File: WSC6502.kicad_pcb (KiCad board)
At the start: 2 copper layers, 145.6 x 157 mm, 43 parts, among them IC1 W65C02S6TPG-14 CPU, IC2 AT28C256-15PU ROM, IC3 AS6C62256-55PCN SRAM, IC4 W65C22S6TPG-14 I/O, J1 +5V, J2 +5V, J3 Address Bus, J4 Data Bus, J5 R~W~ TP, J6 , SW1 Reset, SW2 , SW3 , SW4 , SW5 , SW6 , U1 74HC00, Y1 1MHz

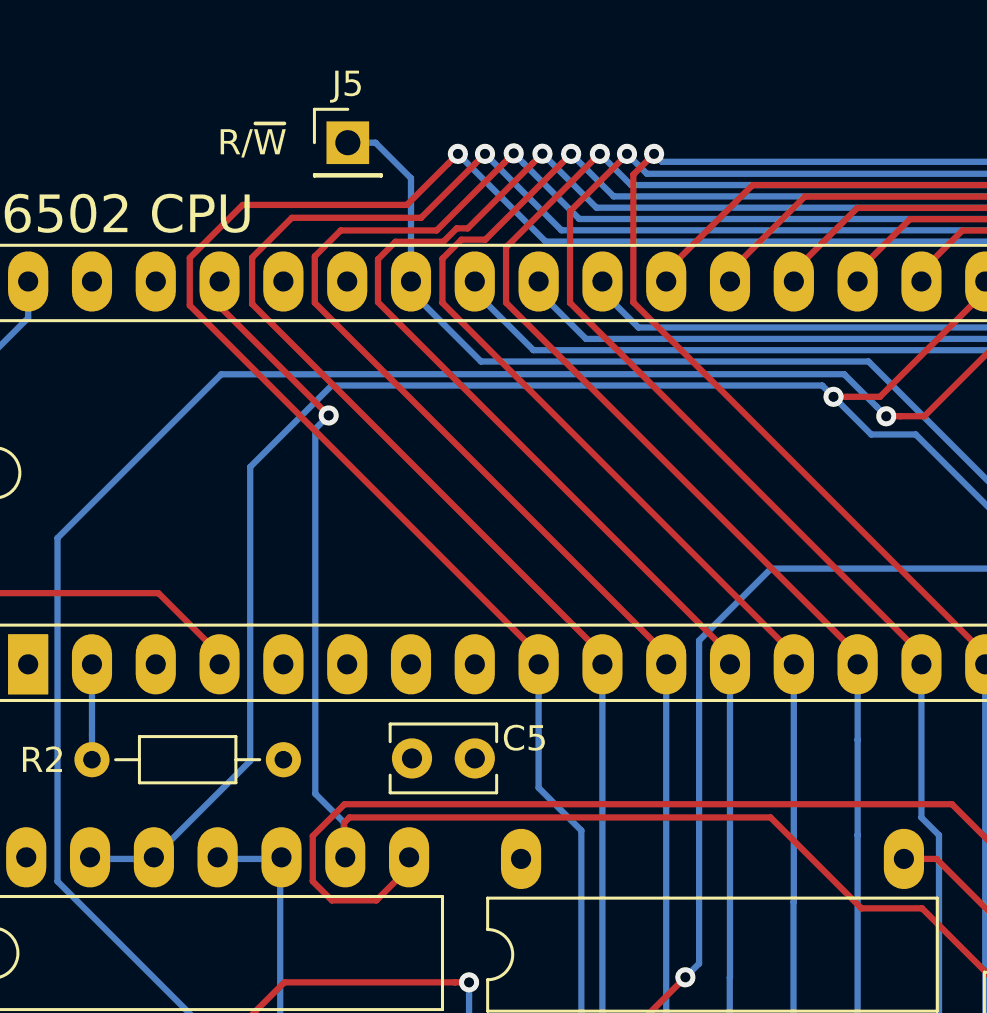
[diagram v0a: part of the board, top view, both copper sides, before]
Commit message: Add files via upload
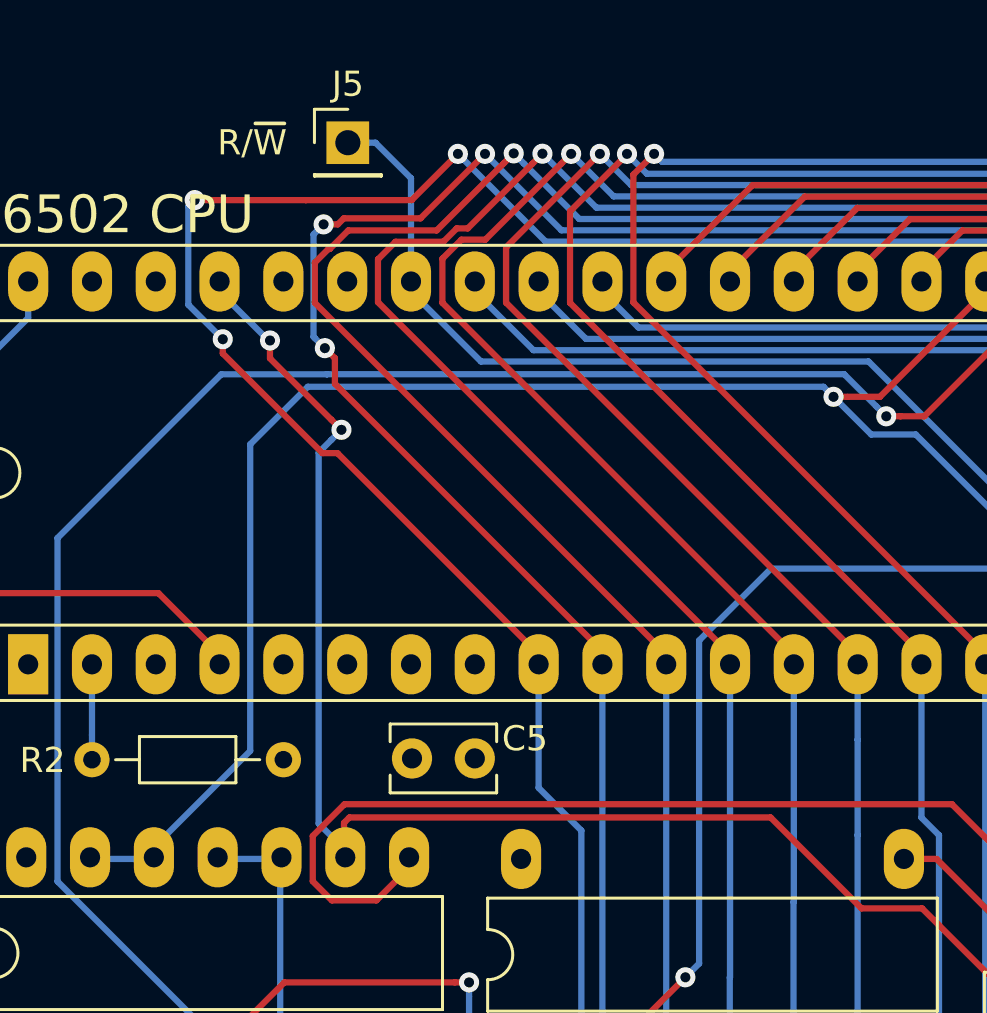
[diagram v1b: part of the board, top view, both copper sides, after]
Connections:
- IC1 pad 36: Net-(IC1-Pad36) -> +5V
- IC1 pad 39: +5V -> Net-(IC1-Pad39)
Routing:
- net /a1: track 184.9 -> 182.0 mm, vias 1 -> 3
- net /a0: track 185.6 -> 187.2 mm, vias 1 -> 3
- net /CLK: track 152.7 -> 153.3 mm, vias 1 -> 2
